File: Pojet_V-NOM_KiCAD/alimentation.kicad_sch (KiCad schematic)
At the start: 17 parts, among them IC401 MP1475SGJ-P

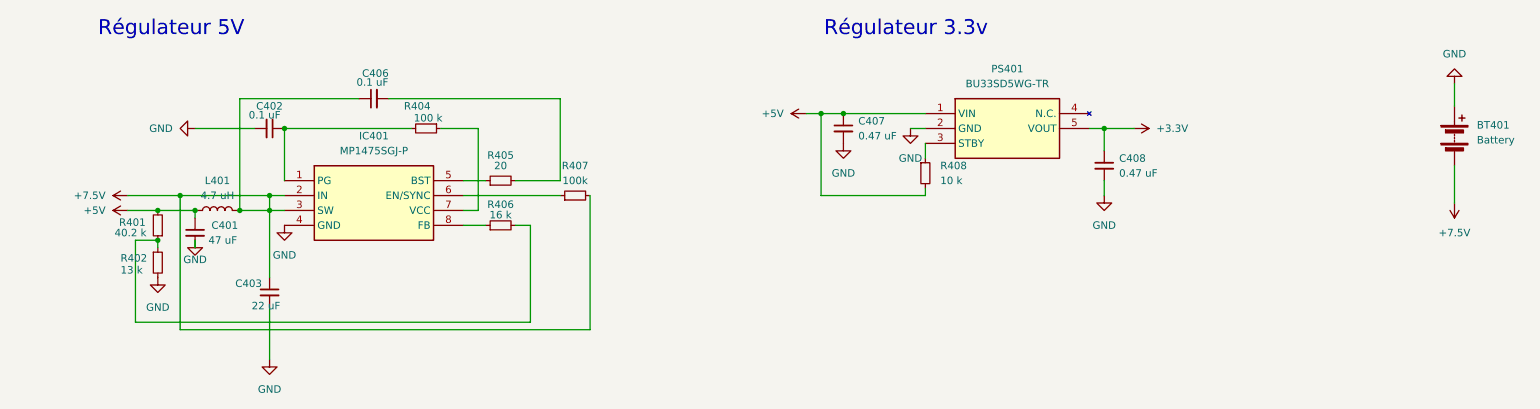
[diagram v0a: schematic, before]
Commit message: regulateur 5 V
Regulateur 5V maj
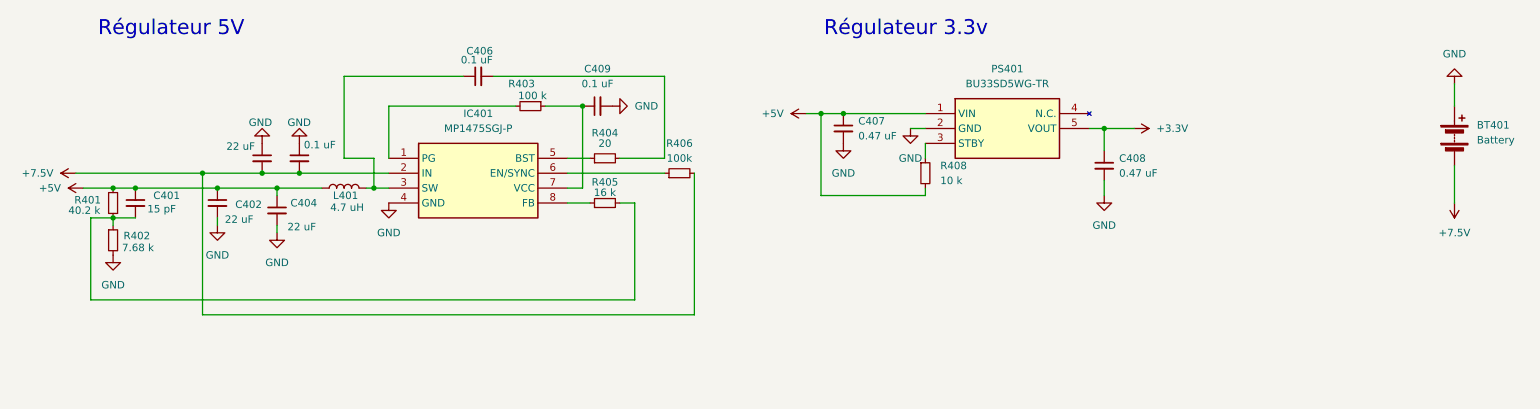
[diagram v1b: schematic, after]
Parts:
- removed R407: 100k, symbol Device:R_Small
- added C404: 22 uF, symbol Device:C_Small
- added C405, C409: 0.1 uF, symbol Device:C_Small
- added R403: 100 k, symbol Device:R_Small
- C401: value 47 uF -> 15 pF
- C402: value 0.1 uF -> 22 uF
- R402: value 13 k -> 7.68 k
- R404: value 100 k -> 20
- R405: value 20 -> 16 k
- R406: value 16 k -> 100k
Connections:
- net +5V: now also C402.1, C404.1
- net +7.5V: now also C403.2, R406.2, C405.2; no longer C403.1, C406.1, IC401.3 (SW), L401.2
- net GND: now also C403.1, C404.2, C405.1, C409.2; no longer C401.2, C403.2
- net at R401.1, R402.1: now also C401.2, R405.2; no longer R406.2
- net at IC401.5 (BST): now also R404.1; no longer R405.1
- net at IC401.6 (EN/SYNC): now also R406.1
- net at IC401.7 (VCC): now also C409.1, R403.1; no longer R404.1
- net at IC401.8 (FB): now also R405.1; no longer R406.1
- net at C406.2: now also R404.2; no longer R405.2
- new net: C406.1, IC401.3 (SW), L401.2
- new net: IC401.1 (PG), R403.2
